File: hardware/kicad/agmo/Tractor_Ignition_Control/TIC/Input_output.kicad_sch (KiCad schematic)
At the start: 28 parts, among them J3 Screw_Terminal_01x04, U17 π140U31, U3 TLP293, U4 TLP293, U6 TLP293

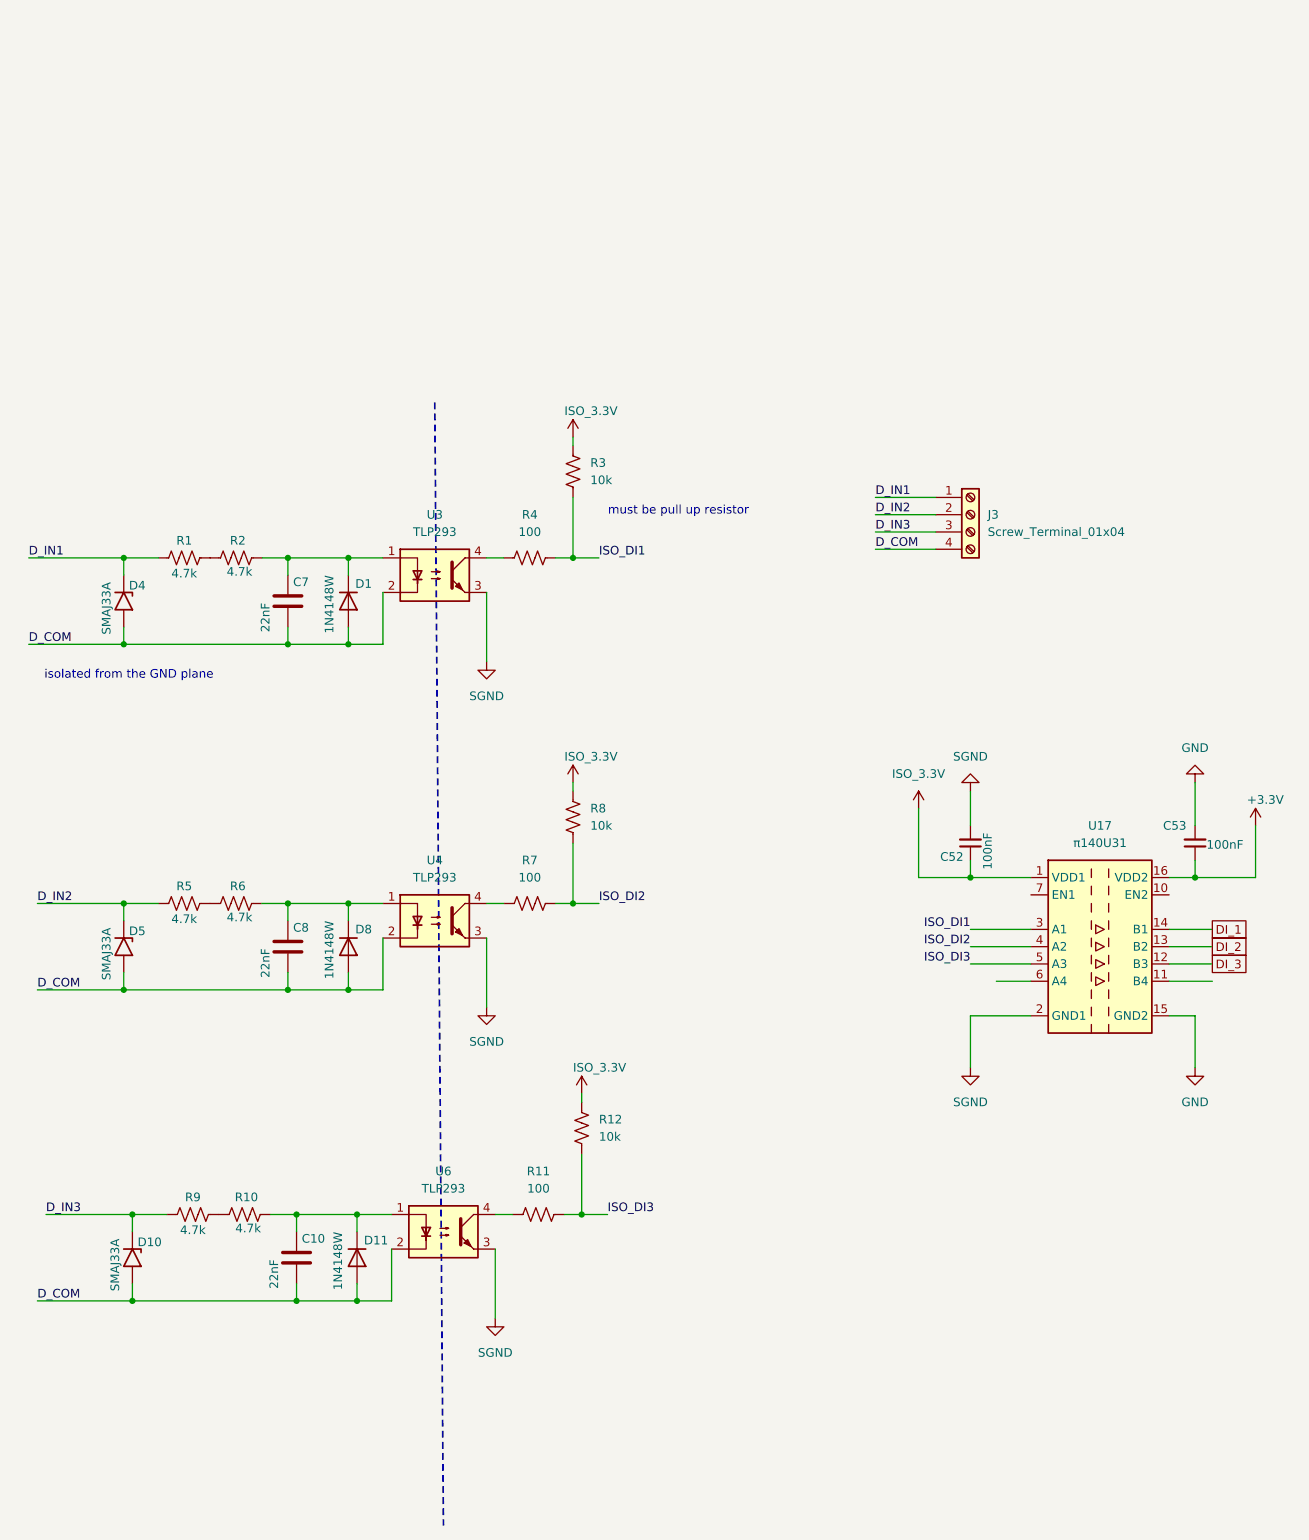
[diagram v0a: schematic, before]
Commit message: feat(hardware): update TIC KiCad design and fabrication files
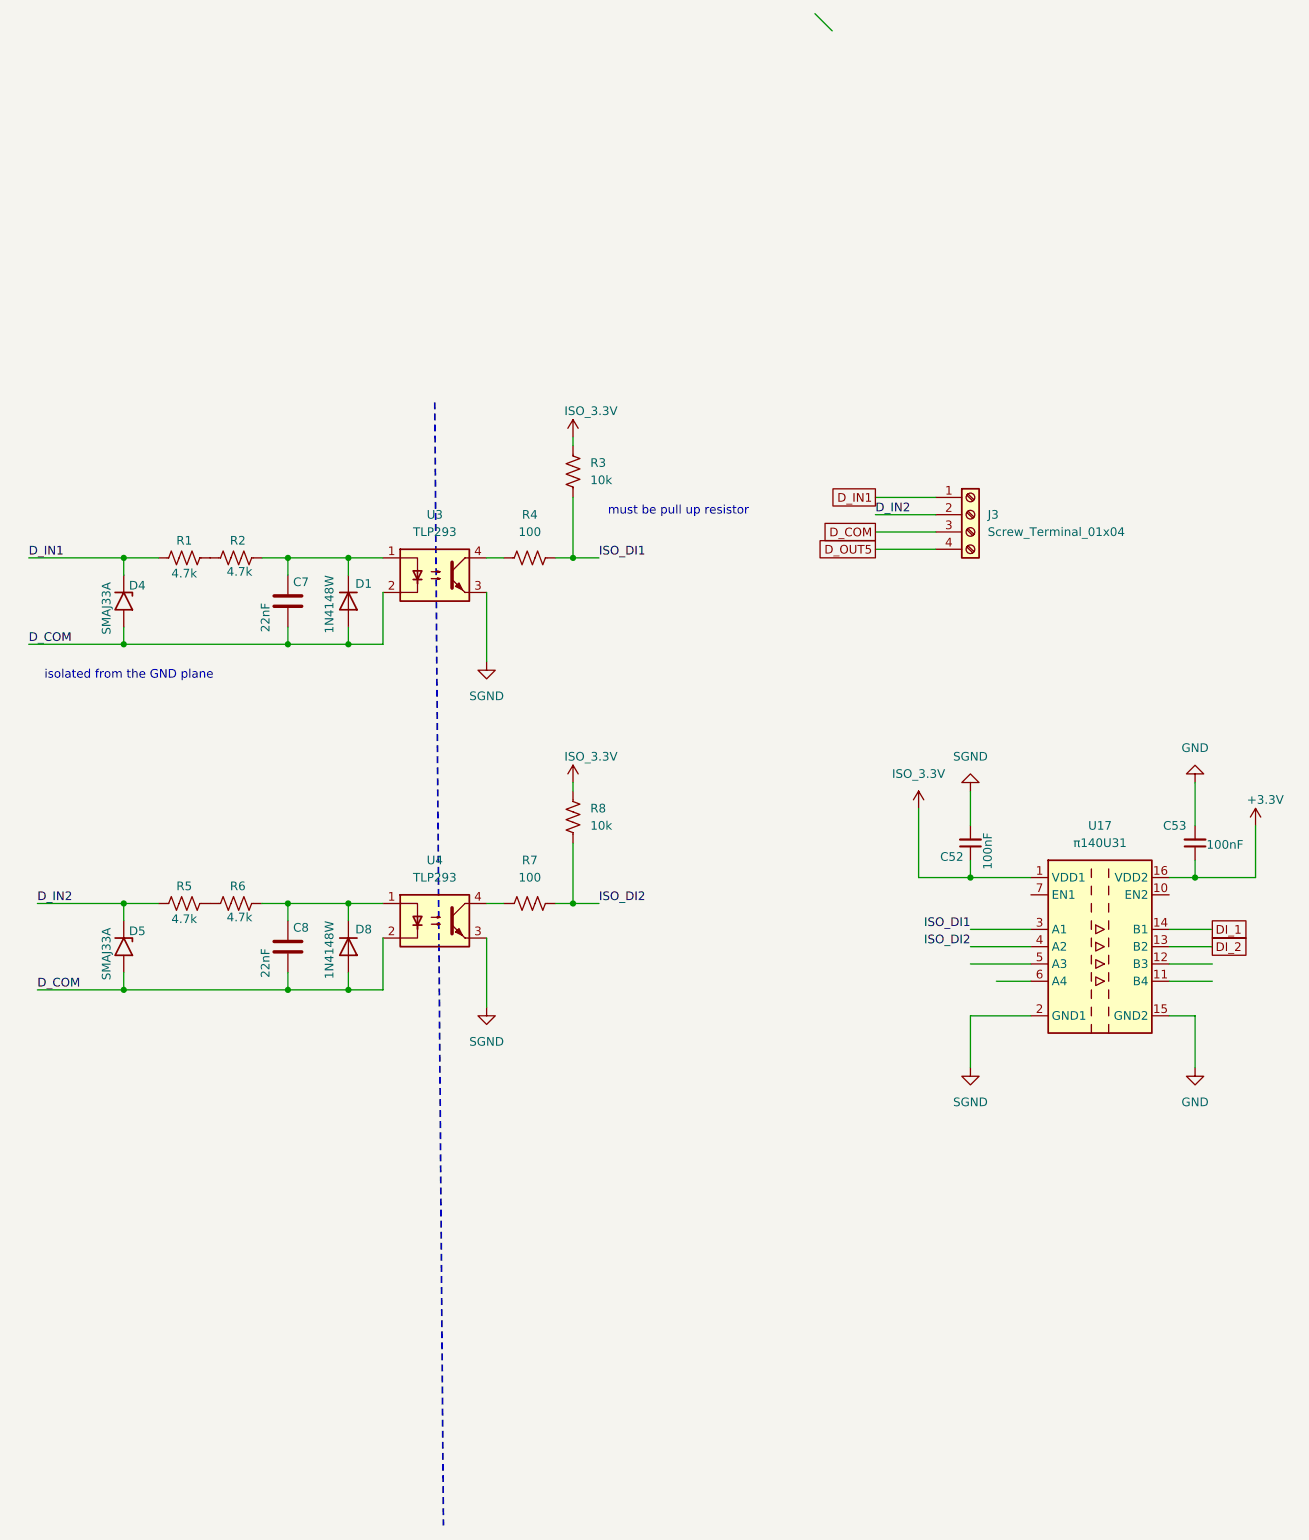
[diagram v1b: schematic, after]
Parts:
- removed C10: 22nF, Capacitor_SMD:C_0805_2012Metric_Pad1.18x1.45mm_HandSolder, symbol Device:C
- removed D10: SMAJ33A, Diode_SMD:D_SMA, symbol Diode:SMAJ33A
- removed D11: 1N4148W, Diode_SMD:D_SOD-123, symbol Diode:1N4148W
- removed R10, R9: 4.7k, Resistor_SMD:R_0805_2012Metric, symbol Device:R_US
- removed R11: 100, Resistor_SMD:R_0805_2012Metric, symbol Device:R_US
- removed R12: 10k, Resistor_SMD:R_0805_2012Metric, symbol Device:R_US
- removed U6: TLP293, Package_SO:SOIC-4_4.55x2.6mm_P1.27mm, symbol Isolator:TLP293
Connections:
- net D_IN3 is gone; now on net D_COM: J3.3 (Pin_3)
- net D_COM: no longer J3.4 (Pin_4)
- net DI_3: no longer names the net of U17.12 (B3)
- net ISO_DI3: no longer names the net of U17.5 (A3)
- new net D_OUT5: J3.4 (Pin_4)
